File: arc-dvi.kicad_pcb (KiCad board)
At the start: 4 copper layers, 94.6 x 71.1 mm, 133 parts, among them J1 Conn_01x24_MountingPin, J2 VIDC Interposer, J3 SWD, J4 BOOT, J5 USB_B_Micro, J6 PWR, Q1 Q_NPN_BCE, U1 W25Q32JVSS, U2 RP2040, U3 ICE40HX4K-TQ144, U4 TDA19988BHN/C1,557, U5 LT1963AxST-3.3, U6 TLV70012_SOT23-5, U7 TLV70018_SOT23-5, Y1 12M 18pF

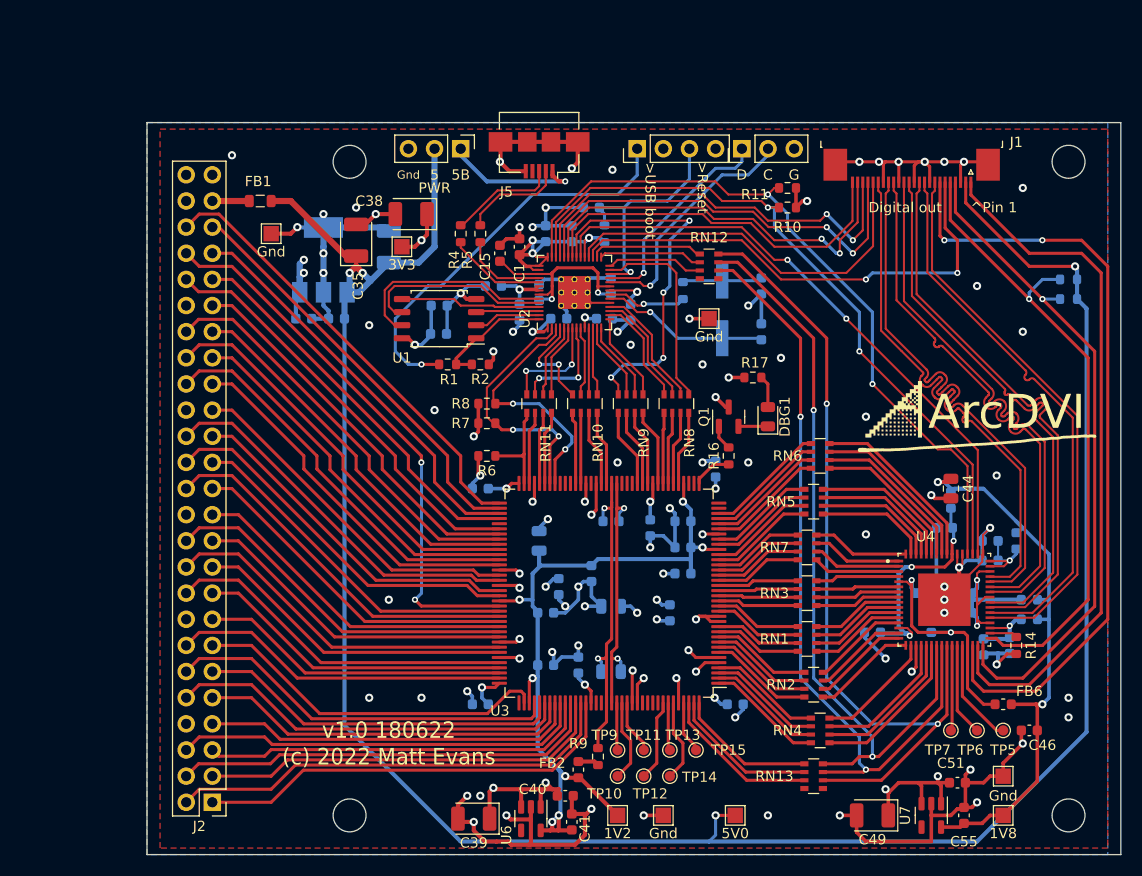
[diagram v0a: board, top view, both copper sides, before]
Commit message: v2: ADV7513 and FFC
Large work much progress - almost routed
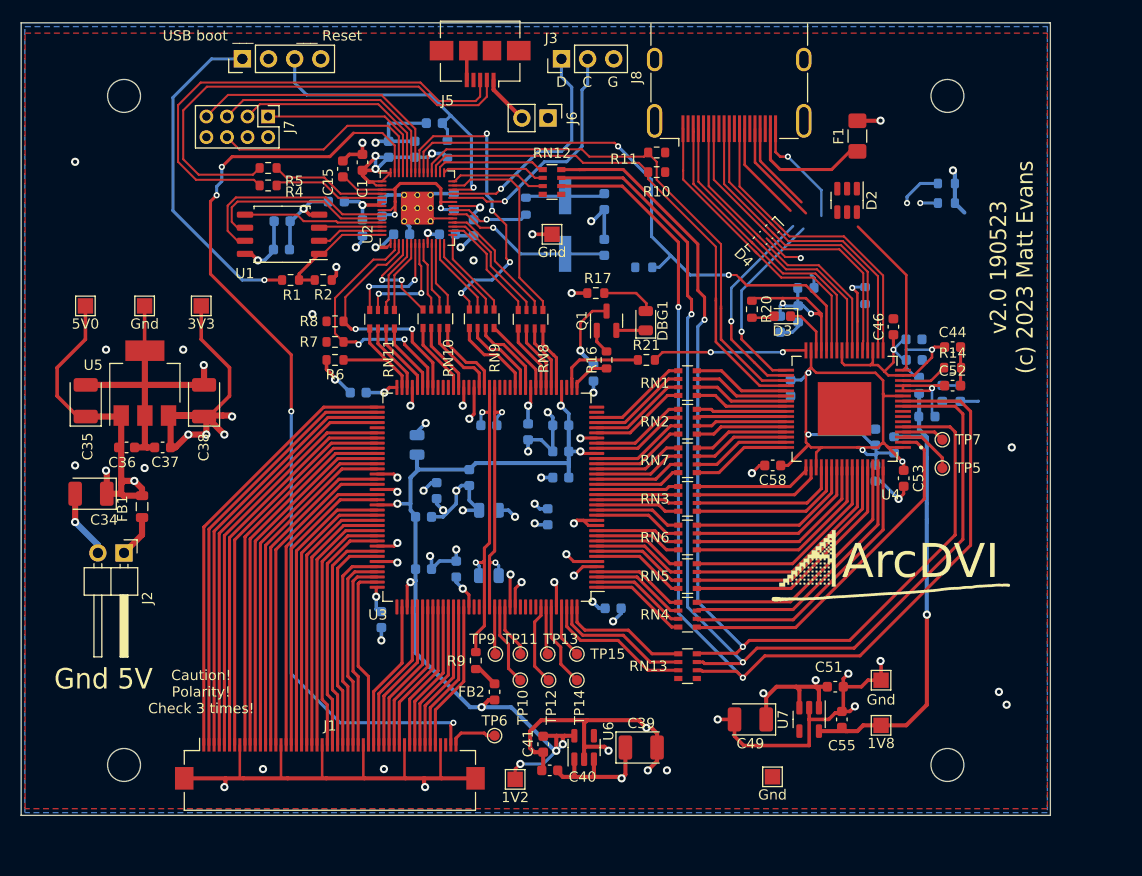
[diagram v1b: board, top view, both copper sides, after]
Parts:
- removed FB6: FerriteBead_Small, Inductor_SMD:L_0603_1608Metric
- added C58: 0.1u, Capacitor_SMD:C_0603_1608Metric, F.Cu at (123.0, 93.0)
- added C59: 0.1u, Capacitor_SMD:C_0603_1608Metric, B.Cu at (124.8, 85.5)
- added D2: ESDA6V1BC6, Package_TO_SOT_SMD:SOT-23-6, F.Cu at (130.2, 67.2)
- added D3: D, Diode_SMD:D_0603_1608Metric, F.Cu at (124.0, 78.5)
- added D4: RCLAMP3328P, Package_DFN_QFN:UDFN-9_1.0x3.8mm_P0.5mm, F.Cu at (122.2, 70.8)
- added F1: 50mA, Fuse:Fuse_1206_3216Metric_Pad1.42x1.75mm_HandSolder, F.Cu at (131.2, 61.0)
- added J7: Misc, Connector_PinHeader_2.00mm:PinHeader_2x04_P2.00mm_Vertical, F.Cu at (74.0, 59.1)
- added J8: HDMI_A, Connector_HDMI:HDMI_A_Molex_208658-1001_Horizontal, F.Cu at (118.8, 57.0)
- added R18: 2K, Resistor_SMD:R_0603_1608Metric, B.Cu at (132.0, 76.5)
- added R19: 2K, Resistor_SMD:R_0603_1608Metric, B.Cu at (110.5, 73.8)
- added R20: 27K, Resistor_SMD:R_0603_1608Metric, F.Cu at (121.0, 77.8)
- added R21: 22, Resistor_SMD:R_0603_1608Metric, F.Cu at (110.8, 82.8)
- C34, C36, C37, C53, U5: moved to F.Cu
- C42: value 1u -> 10u
- C44: value 10u -> 0.1u; footprint Capacitor_SMD:C_0805_2012Metric -> Capacitor_SMD:C_0603_1608Metric
- C46: value 1u -> 0.1u
- C52: value 1u -> 0.1u; moved to F.Cu
- J1: value Conn_01x24_MountingPin -> Connector_50pin_FFC; footprint Connector_FFC-FPC:TE_2-1734839-4_1x24-1MP_P0.5mm_Horizontal -> Connector_FFC-FPC:Hirose_FH12-50S-0.5SH_1x50-1MP_P0.50mm_Horizontal
- J2: value VIDC Interposer -> 5V_IN; footprint Connector_PinHeader_2.54mm:PinHeader_2x25_P2.54mm_Vertical -> Connector_PinHeader_2.54mm:PinHeader_1x02_P2.54mm_Horizontal
- J6: value PWR -> PWR_USB; footprint Connector_PinHeader_2.54mm:PinHeader_1x03_P2.54mm_Vertical -> Connector_PinHeader_2.54mm:PinHeader_1x02_P2.54mm_Vertical
- R12, R13: value 10K -> 2K
- R14: value 10K, 1% -> 887, 1%
- R16: value 4k7 -> 4K7
- TP5: value AP4 -> SPD
- TP6: value AP3 -> P50
- TP7: value AP2 -> MCLK
- U4: value TDA19988BHN/C1,557 -> ADV7513BSWZ; footprint matt:QFN50P900X900X100-65N -> matt:QFP50P1200X1200X160-65N
- moved J1 80.9 mm to (80.0, 122.0), turned to 0 degrees
- moved TP1 80.2 mm to (56.2, 77.5)
- moved TP6 46.9 mm to (96.0, 119.2)
- moved C46 41.4 mm to (134.8, 79.5), turned to 90 degrees
- moved J4 39.3 mm to (71.5, 53.5)
- moved C34 37.6 mm to (56.8, 95.8), turned to 180 degrees
- moved FB1 31.8 mm to (61.8, 97.0), turned to -90 degrees
- moved C56 31.3 mm to (123.8, 79.3), turned to -90 degrees
- moved C42 30.6 mm to (136.8, 80.8), turned to 0 degrees
- moved C35 30.6 mm to (56.3, 86.7)
- moved C43 29.2 mm to (136.8, 82.8), turned to 0 degrees
- moved RN2 28.3 mm to (114.8, 88.8)
- moved TP7 28.3 mm to (139.5, 90.5)
- moved R14 27.7 mm to (140.5, 83.5), turned to 0 degrees
- moved RN1 27.4 mm to (114.8, 85.0)
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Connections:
- C42 pad 1: /Video/VDDA -> /Video/AVDD
- C43 pad 1: /Video/VDDA -> /Video/AVDD
- C44 pad 1: +1V8 -> /Video/AVDD
- C45 pad 1: /Video/VDDA_TX -> /Video/PVDD
- C46 pad 1: +1V8 -> /Video/AVDD
- C47 pad 1: /Video/VDDA_TX -> /Video/PVDD
- C48 pad 1: /Video/VDDA_PLL -> /Video/DVDD
- C50 pad 1: /Video/VDDA_PLL -> /Video/DVDD
- C52 pad 1: /Video/VDD_CORE -> /Video/PVDD
- C53 pad 1: /Video/VDD_CORE -> /Video/DVDD
- C54 pad 1: /Video/VDD_IO -> /Video/DVDD3
- C56 pad 1: /Video/VDD_IO -> /Video/DVDD3
- FB1 pad 2: /HOST_5V -> Net-(FB1-Pad2)
- FB3 pad 2: /Video/VDDA -> /Video/AVDD
- FB4 pad 2: /Video/VDDA_TX -> /Video/PVDD
- FB5 pad 2: /Video/VDDA_PLL -> /Video/DVDD
- FB7 pad 1: +1V8 -> +3V3
- FB7 pad 2: /Video/VDD_IO -> /Video/DVDD3
- J1 pad 1: VID_HPD -> VD0
- J1 pad 10: VID_CK+ -> VD8
- J1 pad 11: VID_D0- -> VD9
- J1 pad 12: GND -> VD10
- J1 pad 13: VID_D0+ -> VD11
- J1 pad 14: VID_D1- -> VD12
- J1 pad 15: GND -> VD13
- J1 pad 16: VID_D1+ -> GND
- J1 pad 17: VID_D2- -> VD14
- J1 pad 18: GND -> VD15
- J1 pad 19: VID_D2+ -> VD16
- J1 pad 2: +5V -> VD1
- J1 pad 20: CFG_SW3 -> VD17
- J1 pad 21: CFG_SW2 -> VD18
- J1 pad 22: CFG_SW1 -> VD19
- J1 pad 23: MCU_A2 -> VD20
- J1 pad 24: MCU_A1 -> GND
- J1 pad 3: GND -> VD2
- J1 pad 4: VID_DISP_SDA -> VD3
- J1 pad 5: VID_DISP_SCL -> VD4
- J1 pad 6: CFG_SW4 -> VD5
- J1 pad 7: VID_CEC -> VD6
- J1 pad 8: VID_CK- -> GND
- J1 pad 9: GND -> VD7
- J2 pad 1: VD15 -> Net-(FB1-Pad2)
- J2 pad 2: VD14 -> GND
- J6 pad 1: /VBUS -> +5V
- J6 pad 2: +5V -> /VBUS
- R12 pad 2: VID_DISP_SDA -> /Video/DDC_SDA
- R13 pad 2: VID_DISP_SCL -> /Video/DDC_SCL
- RN1 pad 1: RGB8 -> RGB23
- RN1 pad 2: RGB23 -> RGB22
- RN1 pad 3: RGB22 -> RGB21
- RN1 pad 4: RGB21 -> RGB20
- RN13 pad 1: ALT_VID_I2S_CLK -> ALT_VID_I2S_DATA
- RN13 pad 2: ALT_VID_I2S_WS -> ALT_VID_I2S_CLK
- RN13 pad 3: ALT_VID_I2S_DATA -> ALT_VID_I2S_WS
- RN13 pad 6: Net-(RN12-Pad8) -> Net-(RN12-Pad6)
- RN13 pad 7: Net-(RN12-Pad6) -> Net-(RN12-Pad7)
- RN13 pad 8: Net-(RN12-Pad7) -> Net-(RN12-Pad8)
- RN2 pad 1: RGB20 -> RGB19
- RN2 pad 2: RGB19 -> RGB18
- RN2 pad 3: RGB18 -> RGB17
- RN2 pad 4: RGB17 -> RGB16
- RN3 pad 1: VID_OUT_PCLK -> RGB11
- RN3 pad 2: RGB11 -> RGB10
- RN3 pad 3: RGB10 -> RGB9
- RN3 pad 4: RGB9 -> VID_OUT_PCLK
- RN3 pad 8: /Video/PCLK_R -> Net-(RN3-Pad8)
- RN4 pad 1: RGB16 -> RGB0
- RN4 pad 3: VID_OUT_VS -> VID_OUT_HS
- RN4 pad 4: VID_OUT_HS -> VID_OUT_VS
- RN4 pad 5: Net-(RN4-Pad5) -> Net-(U4-Pad2)
- RN4 pad 6: Net-(RN4-Pad6) -> Net-(U4-Pad64)
- RN4 pad 7: Net-(RN4-Pad7) -> Net-(U4-Pad63)
- RN4 pad 8: Net-(RN4-Pad8) -> Net-(U4-Pad62)
- RN5 pad 1: RGB3 -> RGB4
- RN5 pad 2: RGB2 -> RGB3
- RN5 pad 3: RGB1 -> RGB2
- RN5 pad 4: RGB0 -> RGB1
- RN6 pad 1: RGB7 -> RGB8
- RN6 pad 2: RGB6 -> RGB7
- RN6 pad 3: RGB5 -> RGB6
- RN6 pad 4: RGB4 -> RGB5
- TP6 pad 1: Net-(TP6-Pad1) -> Net-(J1-Pad50)
- U2 pad 31: CFG_SW4 -> MCU_VID_SDA
- U2 pad 32: CFG_SW3 -> MCU_VID_SCL
- U2 pad 36: MCU_A1 -> /MCU/spare24
- U2 pad 37: MCU_A2 -> /MCU/spare25
- U2 pad 38: CFG_SW2 -> /MCU/spare26
- U2 pad 39: CFG_SW1 -> /MCU/spare27
- U2 pad 40: MCU_VID_SDA -> /MCU/spare28
- U2 pad 41: MCU_VID_SCL -> ID_DET
- U3 pad 1: VID_OUT_HS -> VID_OUT_VS
- U3 pad 10: RGB20 -> RGB4
- U3 pad 101: VD30 -> VD23
- U3 pad 102: VD31 -> VD24
- U3 pad 104: VD0 -> VD25
- U3 pad 105: VD1 -> VD26
- U3 pad 106: VD2 -> VD27
- U3 pad 107: VD3 -> VD28
- U3 pad 11: RGB21 -> RGB5
- U3 pad 110: VD4 -> VD29
- U3 pad 112: VD5 -> VD30
- U3 pad 113: VD6 -> VD31
- U3 pad 114: VD7 -> VnVIDW
- U3 pad 115: VD8 -> VnHS
- U3 pad 116: VD9 -> VnVCS
- U3 pad 117: VD10 -> VnVIDRQ
- U3 pad 118: VD11 -> VnSNDRQ
- U3 pad 119: VD12 -> VFLYBK
- U3 pad 12: RGB22 -> RGB6
- U3 pad 120: VD13 -> VCKIN
- U3 pad 121: VD14 -> VVIDAK
- U3 pad 122: VD15 -> VSNDAK
- U3 pad 142: ALT_VID_I2S_DATA -> ALT_VID_I2S_WS
- U3 pad 143: ALT_VID_I2S_WS -> ALT_VID_I2S_CLK
- U3 pad 144: ALT_VID_I2S_CLK -> ALT_VID_I2S_DATA
- U3 pad 15: RGB23 -> RGB7
- U3 pad 17: RGB9 -> VID_OUT_PCLK
- U3 pad 18: RGB10 -> RGB9
- U3 pad 19: RGB11 -> RGB10
- U3 pad 2: VID_OUT_VS -> VID_OUT_HS
- U3 pad 20: VID_OUT_PCLK -> RGB11
- U3 pad 25: RGB0 -> RGB16
- U3 pad 26: RGB1 -> RGB17
- U3 pad 28: RGB2 -> RGB18
- U3 pad 29: RGB3 -> RGB19
- U3 pad 31: RGB4 -> RGB20
- U3 pad 32: RGB5 -> RGB21
- U3 pad 33: RGB6 -> RGB22
- U3 pad 34: RGB7 -> RGB23
- U3 pad 38: unconnected-(U3-Pad38) -> VID_CEC_CLK
- U3 pad 4: RGB16 -> RGB0
- U3 pad 7: RGB17 -> RGB1
- U3 pad 73: VVIDAK -> VD0
- U3 pad 74: VSNDAK -> VD1
- U3 pad 75: VFLYBK -> VD2
- U3 pad 76: VnSNDRQ -> VD3
- U3 pad 78: VnVIDRQ -> VD4
- U3 pad 79: VnHS -> VD5
- U3 pad 8: RGB18 -> RGB2
- U3 pad 80: VnVCS -> VD6
- U3 pad 81: VnVIDW -> VD7
- U3 pad 82: VD16 -> VD8
- U3 pad 83: VD17 -> VD9
- U3 pad 84: VD18 -> VD10
- U3 pad 85: VD19 -> VD11
- U3 pad 87: VD20 -> VD12
- U3 pad 88: VD21 -> VD13
- U3 pad 9: RGB19 -> RGB3
- U3 pad 90: VD22 -> VD14
- U3 pad 91: VD23 -> VD15
- U3 pad 93: VCKIN -> VD16
- U3 pad 94: VD24 -> VD17
- U3 pad 95: VD25 -> VD18
- U3 pad 96: VD26 -> VD19
- U3 pad 97: VD27 -> VD20
- U3 pad 98: VD28 -> VD21
- U3 pad 99: VD29 -> VD22
- U4 pad 1: Net-(RN7-Pad7) -> /Video/DVDD
- U4 pad 10: Net-(RN1-Pad7) -> Net-(RN12-Pad6)
- U4 pad 11: Net-(RN1-Pad6) -> /Video/DVDD
- U4 pad 12: Net-(RN1-Pad5) -> /Video/PVDD
- U4 pad 13: Net-(RN2-Pad8) -> /Video/PVDD
- U4 pad 14: /Video/VDD_IO -> Net-(R14-Pad1)
- U4 pad 15: Net-(RN2-Pad7) -> /Video/AVDD
- U4 pad 16: Net-(RN2-Pad6) -> /Video/HPD
- U4 pad 17: Net-(RN2-Pad5) -> /Video/TXC-
- U4 pad 18: Net-(RN4-Pad8) -> /Video/TXC+
- U4 pad 19: GND -> /Video/AVDD
- U4 pad 2: Net-(RN7-Pad6) -> Net-(U4-Pad2)
- U4 pad 20: Net-(RN4-Pad7) -> /Video/TX0-
- U4 pad 21: Net-(RN4-Pad6) -> /Video/TX0+
- U4 pad 22: Net-(RN4-Pad5) -> Net-(R18-Pad1)
- U4 pad 23: Net-(RN12-Pad7) -> /Video/TX1-
- U4 pad 24: Net-(RN12-Pad6) -> /Video/TX1+
- U4 pad 25: Net-(RN12-Pad8) -> /Video/AVDD
- U4 pad 26: Net-(TP7-Pad1) -> /Video/TX2-
- U4 pad 27: Net-(TP6-Pad1) -> /Video/TX2+
- U4 pad 28: Net-(TP5-Pad1) -> MCU_VID_IRQ
- U4 pad 29: /Video/VDD_CORE -> /Video/DVDD3
- U4 pad 3: Net-(RN7-Pad5) -> Net-(TP5-Pad1)
- U4 pad 30: VID_CEC -> /Video/CEC
- U4 pad 31: VID_HPD -> /Video/DVDD
- U4 pad 32: VID_DISP_SDA -> Net-(U4-Pad32)
- U4 pad 33: VID_DISP_SCL -> /Video/DDC_SCL
- U4 pad 34: Net-(R14-Pad1) -> /Video/DDC_SDA
- U4 pad 35: /Video/VDDA -> MCU_VID_SCL
- U4 pad 36: /Video/VDDA_TX -> MCU_VID_SDA
- U4 pad 37: VID_CK- -> Net-(RN1-Pad8)
- U4 pad 38: VID_CK+ -> Net-(RN1-Pad7)
- U4 pad 39: VID_D0- -> Net-(RN1-Pad6)
- U4 pad 4: /Video/PCLK_R -> Net-(TP7-Pad1)
- U4 pad 40: VID_D0+ -> Net-(RN1-Pad5)
- U4 pad 41: /Video/VDDA_TX -> Net-(RN2-Pad8)
- U4 pad 42: VID_D1- -> Net-(RN2-Pad7)
- U4 pad 43: VID_D1+ -> Net-(RN2-Pad6)
- U4 pad 44: VID_D2- -> Net-(RN2-Pad5)
- U4 pad 45: VID_D2+ -> Net-(RN7-Pad8)
- U4 pad 46: /Video/VDDA_TX -> Net-(RN7-Pad7)
- U4 pad 47: /Video/VDDA_PLL -> Net-(RN7-Pad6)
- U4 pad 48: /Video/VDDA_PLL -> Net-(RN7-Pad5)
- U4 pad 49: GND -> Net-(RN3-Pad8)
- U4 pad 5: /Video/VDD_CORE -> Net-(RN12-Pad8)
- U4 pad 50: MCU_VID_IRQ -> Net-(RN3-Pad7)
- U4 pad 51: MCU_VID_SDA -> /Video/DVDD
- U4 pad 52: MCU_VID_SCL -> Net-(RN3-Pad6)
- U4 pad 53: GND -> Net-(RN3-Pad5)
- U4 pad 54: GND -> Net-(RN6-Pad8)
- U4 pad 55: /Video/VDD_IO -> Net-(RN6-Pad7)
- U4 pad 56: Net-(RN6-Pad8) -> Net-(RN6-Pad6)
- U4 pad 57: Net-(RN6-Pad7) -> Net-(RN6-Pad5)
- U4 pad 58: Net-(RN6-Pad6) -> Net-(RN5-Pad8)
- U4 pad 59: Net-(RN6-Pad5) -> Net-(RN5-Pad7)
- U4 pad 6: Net-(RN3-Pad7) -> unconnected-(U4-Pad6)
- U4 pad 60: Net-(RN5-Pad8) -> Net-(RN5-Pad6)
- U4 pad 61: Net-(RN5-Pad7) -> Net-(RN5-Pad5)
- U4 pad 62: Net-(RN5-Pad6) -> Net-(U4-Pad62)
- U4 pad 63: Net-(RN5-Pad5) -> Net-(U4-Pad63)
- U4 pad 64: Net-(RN7-Pad8) -> Net-(U4-Pad64)
- U4 pad 7: Net-(RN3-Pad6) -> unconnected-(U4-Pad7)
- U4 pad 8: Net-(RN3-Pad5) -> unconnected-(U4-Pad8)
- U4 pad 9: Net-(RN1-Pad8) -> Net-(RN12-Pad7)
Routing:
- net GND: track 834.2 -> 566.2 mm, vias 85 -> 56
- net +5V: track 225.1 -> 47.8 mm
- net ID_DET: track 0.00 -> 94.3 mm, vias 0 -> 4
- net VID_CEC: track 76.9 -> 0.00 mm, vias 2 -> 0
- net VID_HPD: track 68.1 -> 0.00 mm
- net VID_DISP_SDA: track 64.7 -> 0.00 mm, vias 1 -> 0
- net VID_DISP_SCL: track 61.9 -> 0.00 mm, vias 1 -> 0
- net /Video/DVDD: track 0.00 -> 60.8 mm, vias 0 -> 4
- net VID_CK-: track 54.3 -> 0.00 mm
- net VID_CK+: track 54.3 -> 0.00 mm
- net VID_D0-: track 54.2 -> 0.00 mm
- net VID_D0+: track 54.2 -> 0.00 mm
- net VID_D2-: track 54.2 -> 0.00 mm
- net VID_D2+: track 54.2 -> 0.00 mm
- net VID_D1+: track 54.1 -> 0.00 mm
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- removed copper zone on In1.Cu, net +3V3
- removed copper zone on In2.Cu, net GND
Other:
- board size 94.6 x 71.1 mm -> 100 x 77 mm
- board text added: "Caution! Polarity! Check 3 times!"
- board text added: "Check values of C58 and friends, equal spread pls"
- board text added: "Gnd 5V"
- board text added: "USB boot ___"
- board text added: "___ Reset"
- board text added: "v2.0 190523 (c) 2023 Matt Evans"
- board text removed: "5"
- board text removed: "5B"
- board text removed: ">Reset"
- board text removed: ">USB boot"
- board text removed: "Digital out"
- board text removed: "^Pin 1"
- board text removed: "v1.0 180622 (c) 2022 Matt Evans"
